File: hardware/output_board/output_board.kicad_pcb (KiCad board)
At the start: 2 copper layers, 45 x 17 mm, 7 parts, among them J1 I/O, J2 conn_2x2

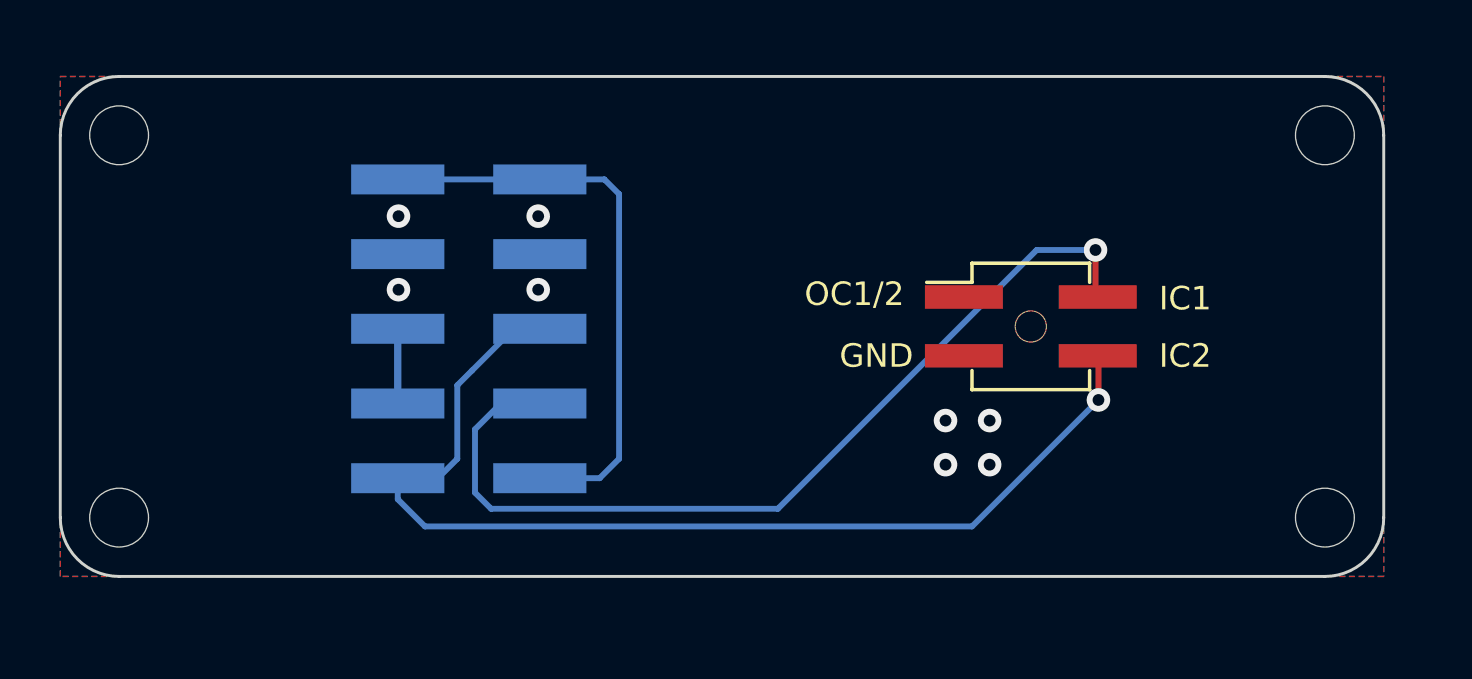
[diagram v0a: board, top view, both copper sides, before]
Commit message: Final refinements
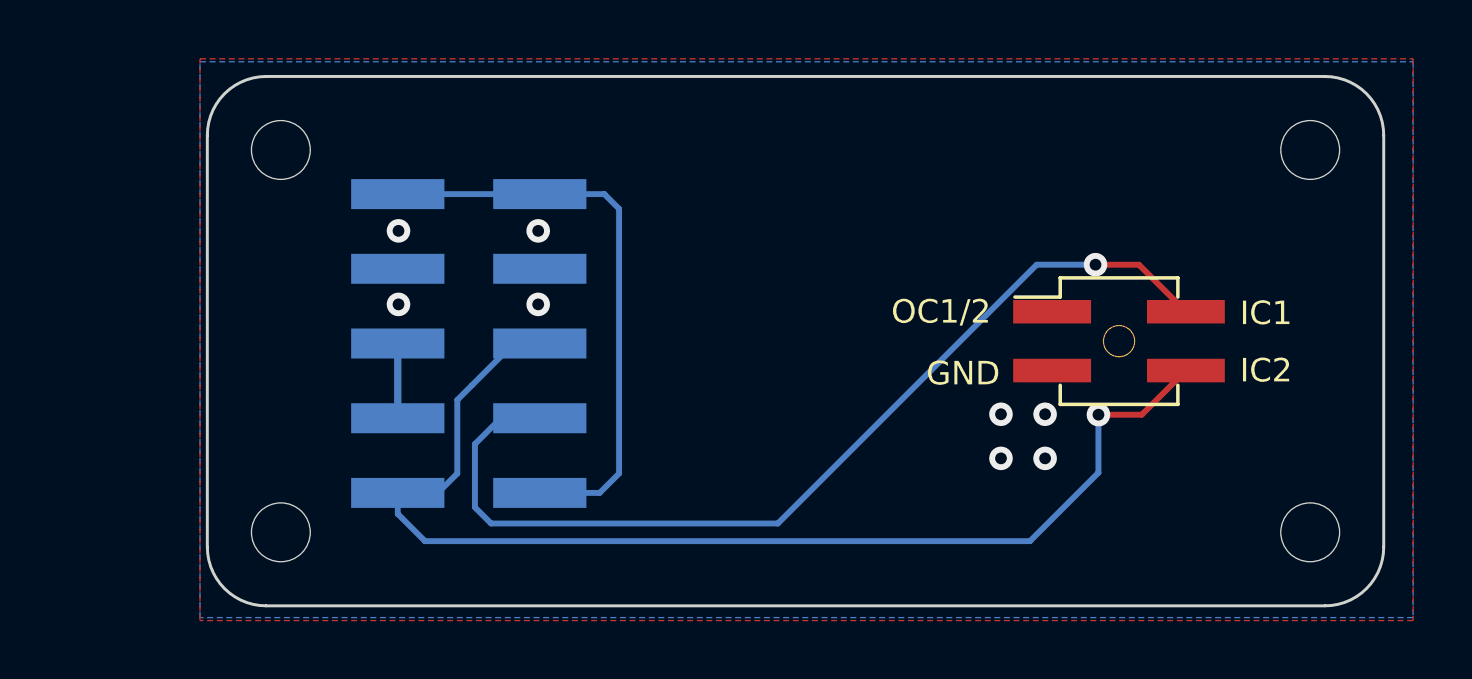
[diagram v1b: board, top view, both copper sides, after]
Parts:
- removed the G*** at (145.2, 108.5)
- added G***: LOGO, cycfi_library:cycfi-logo-9mm, B.Cu at (146.4, 109.0)
- moved H3 5.52 mm to (112.5, 115.5)
- moved H4 5.52 mm to (112.5, 102.5)
- moved J2 3.04 mm to (141.0, 109.0)
- moved H1 0.71 mm to (147.5, 115.5)
- moved H2 0.71 mm to (147.5, 102.5)
- moved J1 0.50 mm to (118.9, 109.1)
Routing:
- net out-: track 36.6 -> 39.9 mm
- net int_coil+: track 31.3 -> 33.4 mm
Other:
- board size 45 x 17 mm -> 40 x 18 mm
